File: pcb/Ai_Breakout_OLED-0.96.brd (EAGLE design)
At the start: 33 x 33 mm, 14 parts, among them J1 2X04, M1 STAND-OFF, M2 STAND-OFF, M3 STAND-OFF, M4 STAND-OFF, U1 UG-2864HSWEG01

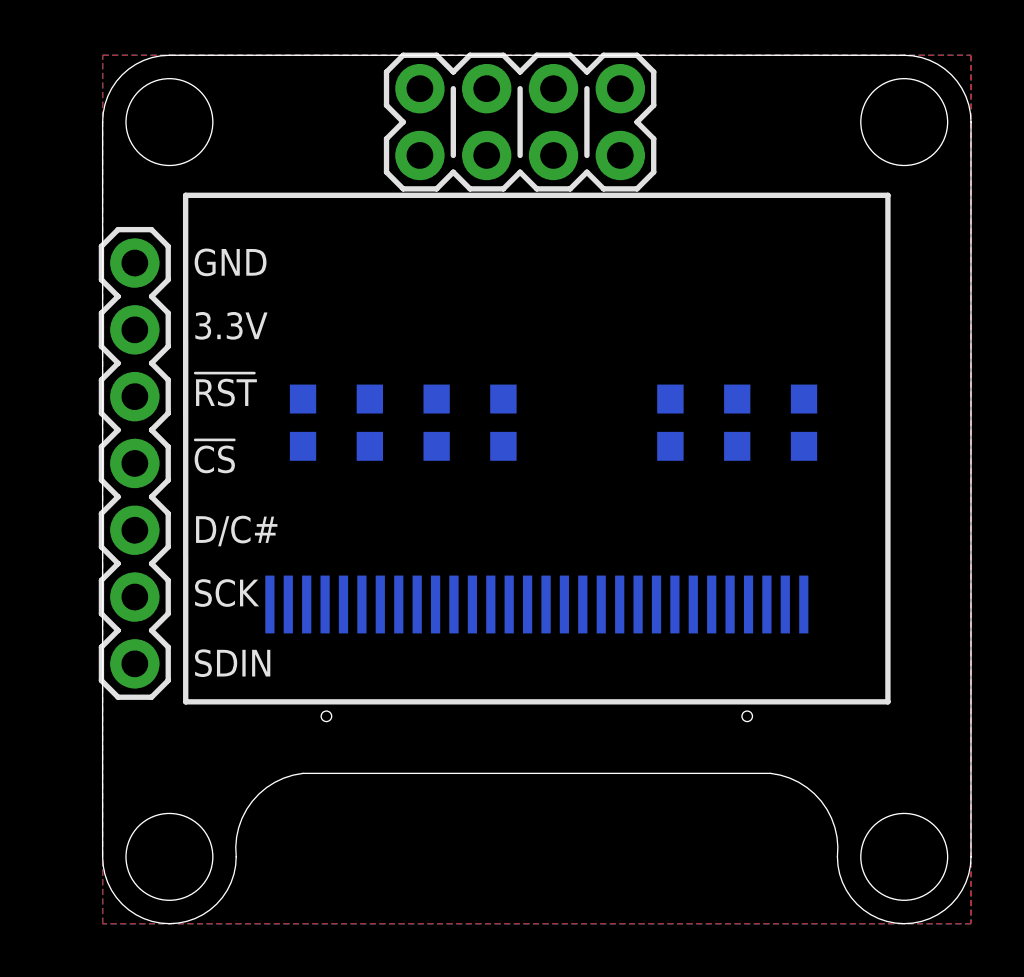
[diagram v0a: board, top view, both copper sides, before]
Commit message: routing done
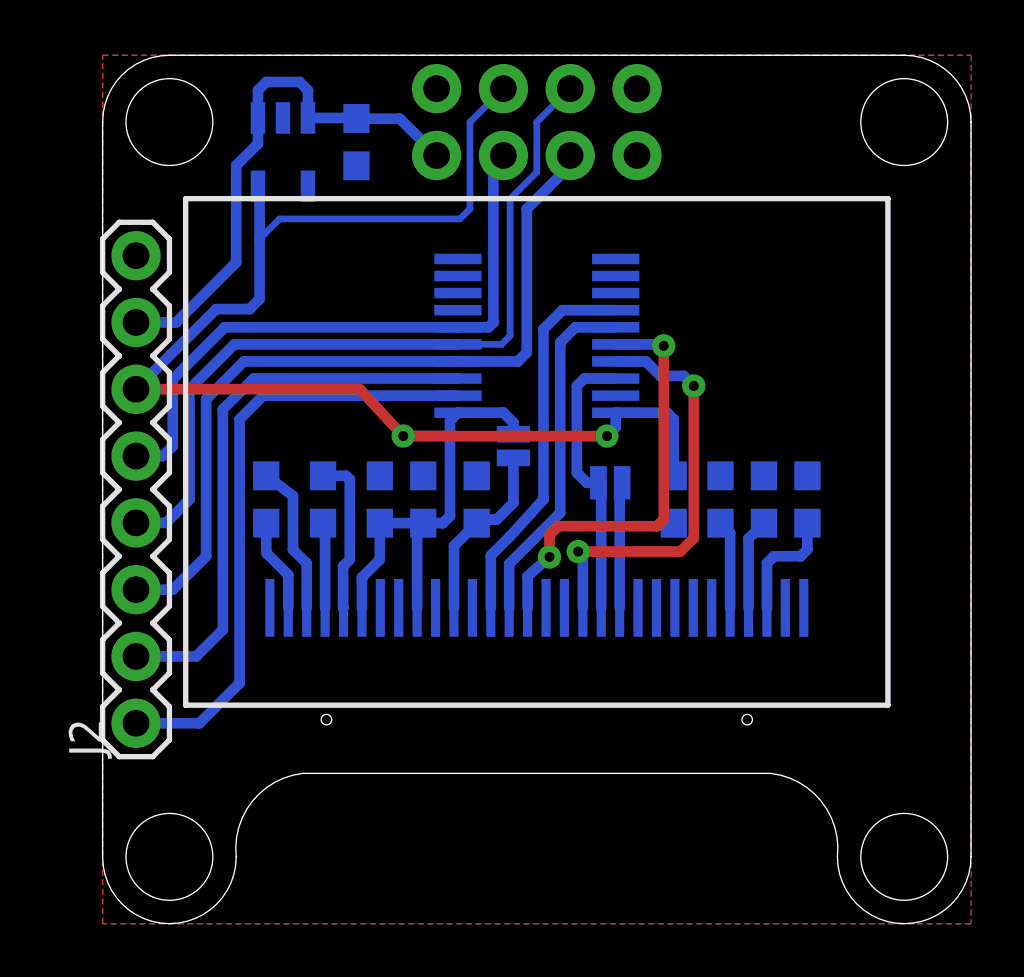
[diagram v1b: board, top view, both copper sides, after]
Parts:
- removed JP1: 1X07, Ai_Connectors:1X07
- added C1, C2: 10uF, Ai_Passives:CAP-0603
- added IC1: 74HCT245MTC, Ai_IC:SSOP20
- added J2: 1X08, Ai_Connectors:1X08
- added JS1, JS2: 1X02-SJ-NO, Ai_Connectors:1X02-SJ-NO
- added R1: 10K, Ai_Passives:RES-0603
- added U2: MIC5205-3.3, Ai_Power:SOT23-5
- C5: value 10uF -> 2.2uF
- C8: value 2.2uF -> 10uF
- moved C5 16.4 mm to (10.5, 16.1)
- moved C7 10.3 mm to (25.1, 16.1)
- moved C8 3.96 mm to (26.8, 16.1)
- moved R3 3.49 mm to (23.5, 16.1)
- moved C4 3.42 mm to (8.38, 16.1)
- moved C3 3.24 mm to (6.22, 16.1)
- moved C6 2.96 mm to (12.2, 16.1)
- moved J1 0.64 mm to (16.5, 30.5), flipped to the bottom
- moved U1 0.13 mm to (16.5, 13.2)
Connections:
- new net CS_IN: IC1.6, J1.5, J2.5
- new net D0/SCLK/SCK_IN: IC1.3, J1.2, J2.2
- new net D1/MOSI/SDA1_IN: IC1.2, J1.1, J2.1
- new net DC/SA0_IN: IC1.4, J1.3, J2.3
- new net I2C_EN: JS2.1, R1.2, U1.11
- new net N$8: JS1.2, U1.20
- new net RST_IN: IC1.5, J1.4, J2.4
- new net VIN: C1.2, J1.7, J2.7, U2.1, U2.3
- net 3V3: now also C2.2, C5.2, IC1.1, IC1.20, J1.6, J2.6, JS2.2, U2.5; no longer C7.2, JP1.6
- net CS_3V3: now also IC1.14; no longer JP1.5
- net D0/SCLK/SCK_3V3: now also IC1.17; no longer JP1.2
- net D1/MOSI/SDA1_3V3: now also IC1.18, JS1.1; no longer JP1.1
- net DC/SA0_3V3: now also IC1.16; no longer JP1.3
- net GND: now also C1.1, C2.1, IC1.10, IC1.19, J1.8, J2.8, R1.1, U2.2; no longer JP1.7, U1.11
- net N$11: now also C8.2; no longer C5.2
- net N$12: now also C7.2; no longer C8.2
- net RST_3V3: now also IC1.15; no longer JP1.4
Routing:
- net 3V3: track 0.00 -> 66.5 mm, vias 0 -> 2
- net DC/SA0_IN: track 0.00 -> 30.3 mm
- net RST_IN: track 0.00 -> 30.0 mm
- net CS_IN: track 0.00 -> 23.7 mm
- net D1/MOSI/SDA1_IN: track 0.00 -> 23.3 mm
- net D0/SCLK/SCK_IN: track 0.00 -> 21.5 mm
- net VIN: track 0.00 -> 20.3 mm
- net DC/SA0_3V3: track 0.00 -> 16.2 mm, vias 0 -> 2
- net D0/SCLK/SCK_3V3: track 0.00 -> 16.0 mm, vias 0 -> 2
- net CS_3V3: track 0.00 -> 14.4 mm
- net RST_3V3: track 0.00 -> 13.2 mm
- net D1/MOSI/SDA1_3V3: track 0.00 -> 10.7 mm
- net I2C_EN: track 0.00 -> 7.01 mm
- net N$7: track 0.00 -> 6.07 mm
- net N$5: track 0.00 -> 5.74 mm
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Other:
- board text removed: "1"
- board text removed: "10"
- board text removed: "20"
- board text removed: "30"

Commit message: ready for fabrication
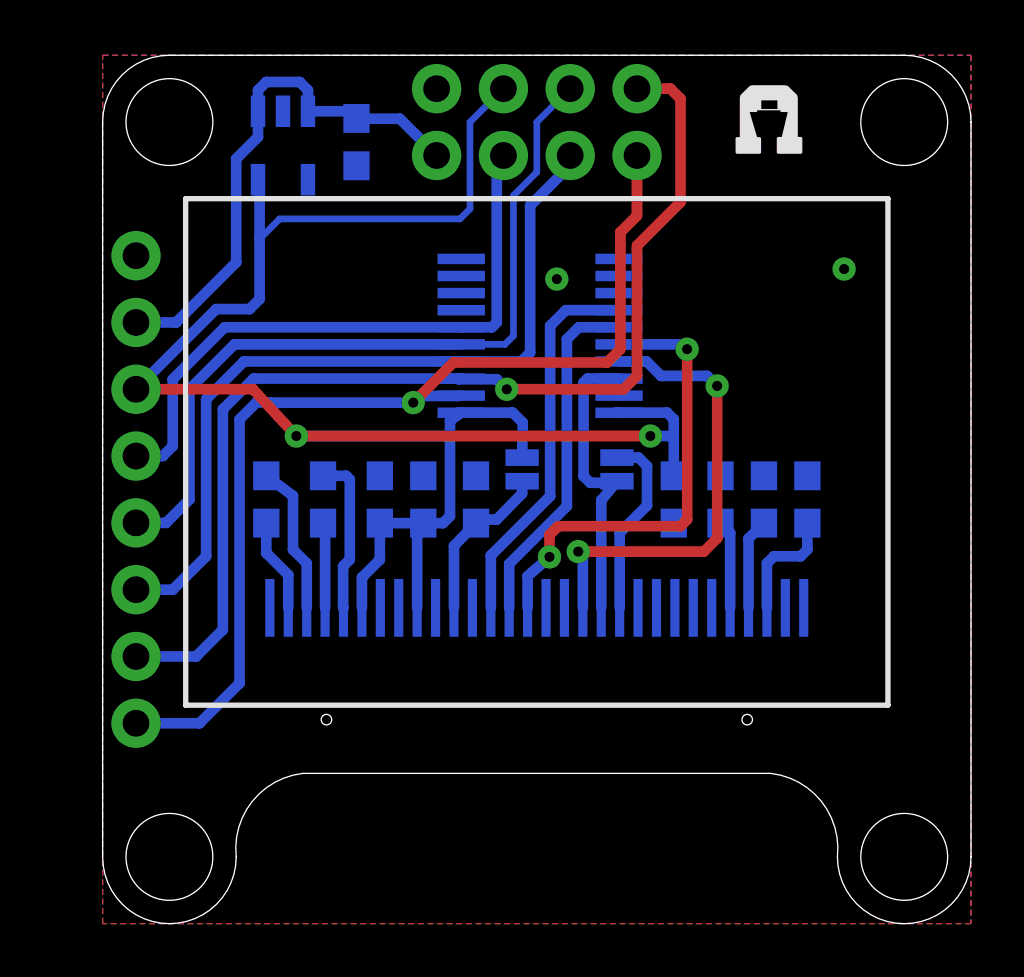
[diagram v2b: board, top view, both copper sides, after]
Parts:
- added U$15, U$16: AI-LOGOXS, Ai_Miscellany:AI-LOGO-XS
- moved JS2 0.95 mm to (16.0, 17.3)
- moved JS1 0.57 mm to (19.6, 17.3), turned to 90 degrees
- moved U2 0.25 mm to (6.86, 29.6)
- moved IC1 0.13 mm to (16.6, 22.4)
- flipped J2 to the bottom
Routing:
- net D0/SCLK/SCK_IN: track 21.5 -> 41.9 mm, vias 0 -> 1
- net D1/MOSI/SDA1_IN: track 23.3 -> 39.7 mm, vias 0 -> 1
- net 3V3: track 66.5 -> 74.0 mm
- net N$8: track 4.79 -> 7.10 mm
- net D0/SCLK/SCK_3V3: track 16.0 -> 17.6 mm
- net DC/SA0_3V3: track 16.2 -> 17.8 mm
- net I2C_EN: track 7.01 -> 6.25 mm
- net D1/MOSI/SDA1_3V3: track 10.7 -> 11.4 mm
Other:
- board text added: "3V3"
- board text added: "D/C"
- board text added: "O: SPI C: I2C"
- board text added: "Pasadena, CA"
- board text added: "UG-2864HSWEG01 BREAKOUT"
- board text added: "VIN"
- board text added: "v1.0"
- board text removed: "3.3V"
- board text removed: "D/C#"
- board text removed: "SSD1306 1.3" 128x64 OLED"
